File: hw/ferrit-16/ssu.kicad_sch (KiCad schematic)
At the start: 40 parts, among them J1 Conn_02x10_Odd_Even, J10 Conn_02x10_Odd_Even, J11 Conn_02x10_Odd_Even, J12 Conn_02x10_Odd_Even, J13 Conn_02x10_Odd_Even, J14 Conn_02x10_Odd_Even, J15 Conn_02x10_Odd_Even, J16 Conn_02x10_Odd_Even, J17 Conn_02x10_Odd_Even, J2 Conn_02x10_Odd_Even, J3 Conn_02x10_Odd_Even, J4 Conn_02x10_Odd_Even, J5 Conn_02x10_Odd_Even, J6 Conn_02x10_Odd_Even, J7 Conn_02x10_Odd_Even, J8 Conn_02x10_Odd_Even, J9 Conn_02x10_Odd_Even, SW3 BOOT, U1 SN74HC154

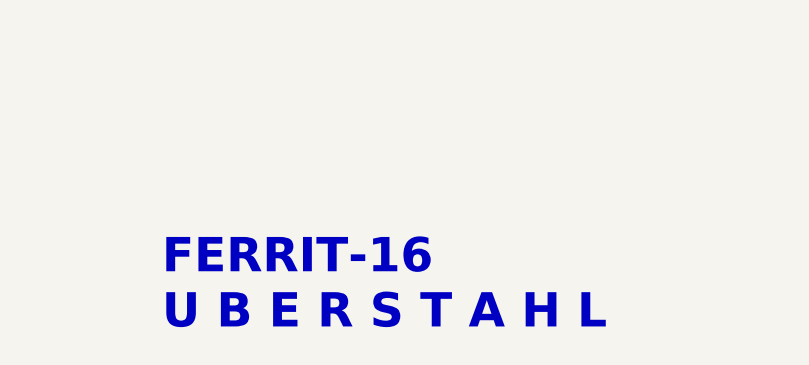
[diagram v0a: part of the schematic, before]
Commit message: cleanup schematics
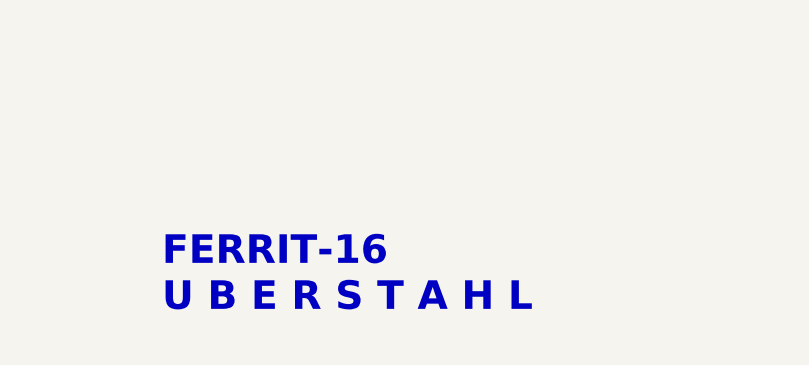
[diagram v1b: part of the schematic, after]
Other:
- company: (none) -> Copyright © 2026 Lone Dynamics Corporation
- title: (none) -> Ferrit -M8 Memory Card (8 x SOP-16)
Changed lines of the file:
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@@
 	(generator_version "8.0")
 	(paper "A1")
+	(title_block
+		(title "Ferrit -M8 Memory Card (8 x SOP-16)")
+		(date "2026-03-07")
+		(rev "V0")
+		(company "Copyright © 2026 Lone Dynamics Corporation")
+	)
 	(wire
 		(pts
@@
 	(text "FERRIT-16\nU B E R S T A H L"
 		(exclude_from_sim no)
-		(at 722.63 563.372 0)
+		(at 722.63 561.34 0)
 		(effects
 			(font
-				(size 3.81 3.81)
+				(size 3.175 3.175)
 				(thickness 1)
 				(bold yes)

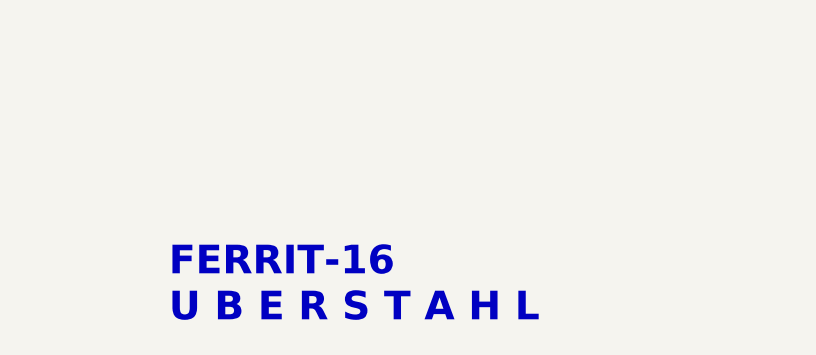
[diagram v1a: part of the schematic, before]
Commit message: cleanup schematics
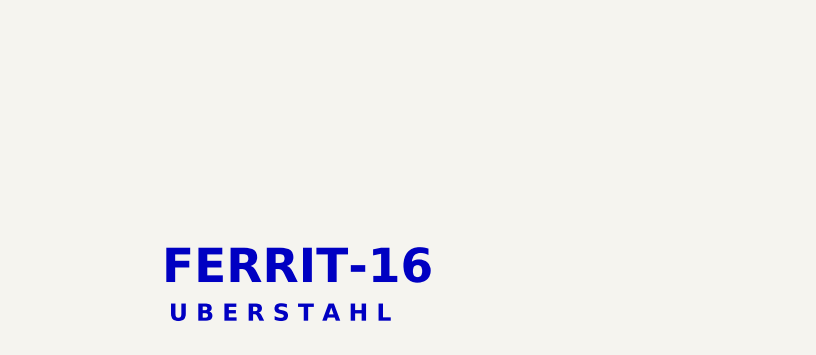
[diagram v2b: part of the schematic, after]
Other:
- note added: "FERRIT-16"
- note added: "U B E R S T A H L"
- note removed: "FERRIT-16 U B E R S T A H L"
- title: Ferrit -M8 Memory Card (8 x SOP-16) -> Ferrit Backplane
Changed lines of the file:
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@@
 	(paper "A1")
 	(title_block
-		(title "Ferrit -M8 Memory Card (8 x SOP-16)")
+		(title "Ferrit Backplane")
 		(date "2026-03-07")
 		(rev "V0")
@@
 		)
 	)
-	(text "FERRIT-16\nU B E R S T A H L"
+	(text "U B E R S T A H L"
 		(exclude_from_sim no)
 		(at 722.63 561.34 0)
 		(effects
 			(font
-				(size 3.175 3.175)
+				(size 1.905 1.905)
+				(thickness 1)
+				(bold yes)
+			)
+			(justify left bottom)
+		)
+	)
+	(text "FERRIT-16"
+		(exclude_from_sim no)
+		(at 721.868 557.276 0)
+		(effects
+			(font
+				(size 3.81 3.81)
 				(thickness 1)
 				(bold yes)
